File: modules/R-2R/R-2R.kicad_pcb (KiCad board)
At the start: 2 copper layers, 40.6 x 40.6 mm, 26 parts, among them J1 Conn_01x10_Male, J2 Conn_01x10_Male, J3 Conn_01x01_Male, J4 Conn_01x01_Male, U1 74LS573

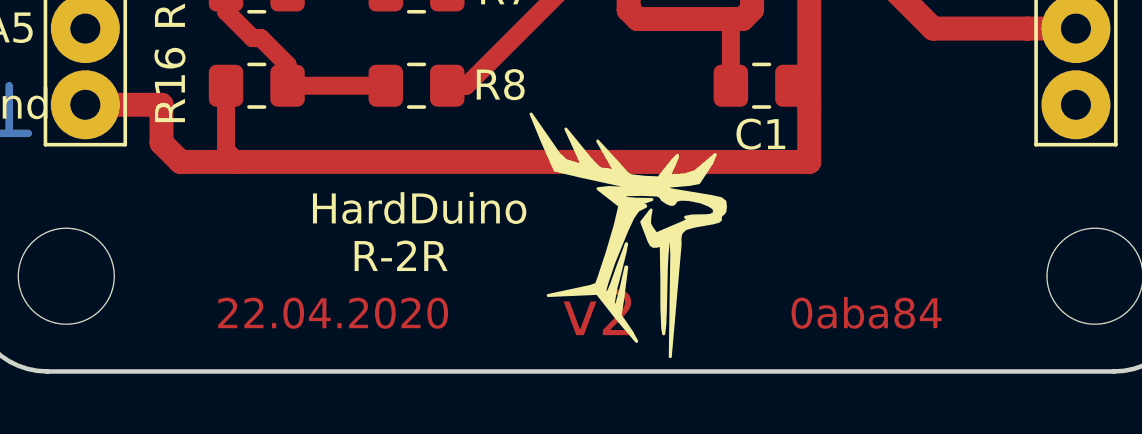
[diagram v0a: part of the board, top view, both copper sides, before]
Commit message: Fix hash & version
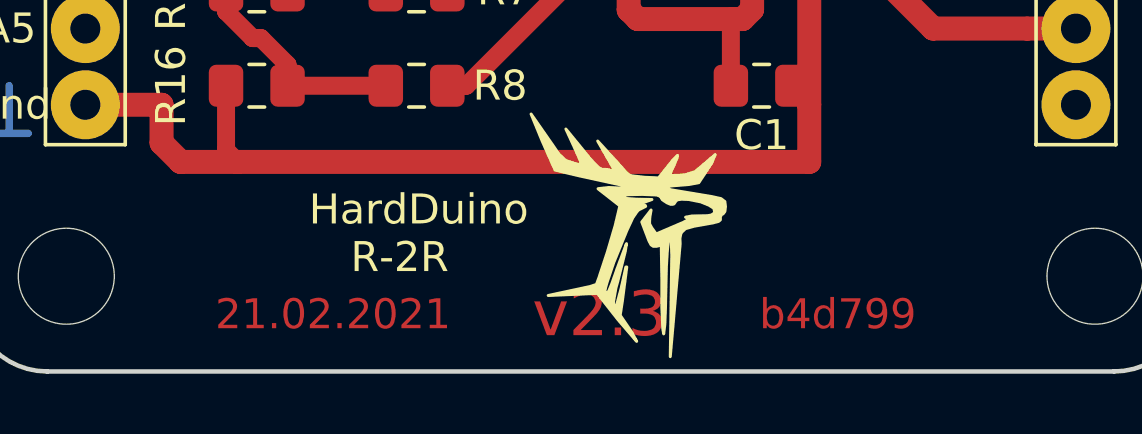
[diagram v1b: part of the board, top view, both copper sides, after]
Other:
- board text added: "21.02.2021"
- board text added: "b4d799"
- board text added: "v2.3"
- board text removed: "0aba84"
- board text removed: "22.04.2020"
- board text removed: "v2"
